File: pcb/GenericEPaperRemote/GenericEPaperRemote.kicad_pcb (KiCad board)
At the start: 2 copper layers, 190.5 x 61 mm, 113 parts, among them J1 Display, J2 speaker, J3 Prog, J4 JTAG, J5 Barrel_Jack, Q1 BC817, Q2 BC817, SW1 TactileSwitchSMD6x6, SW10 TactileSwitchSMD6x6, SW11 Rotary_Encoder_Switch, SW12 reset, SW13 bootloader, SW14 Conn_01x02_Male, SW2 TactileSwitchSMD6x6, SW3 TactileSwitchSMD6x6, SW4 TactileSwitchSMD6x6, SW5 TactileSwitchSMD6x6, SW6 TactileSwitchSMD6x6, SW7 TactileSwitchSMD6x6, SW8 TactileSwitchSMD6x6, SW9 TactileSwitchSMD6x6, U1 ESP32-WROVER-B_(16MB), U2 FT232RL, U3 NCP1117ST33T3G

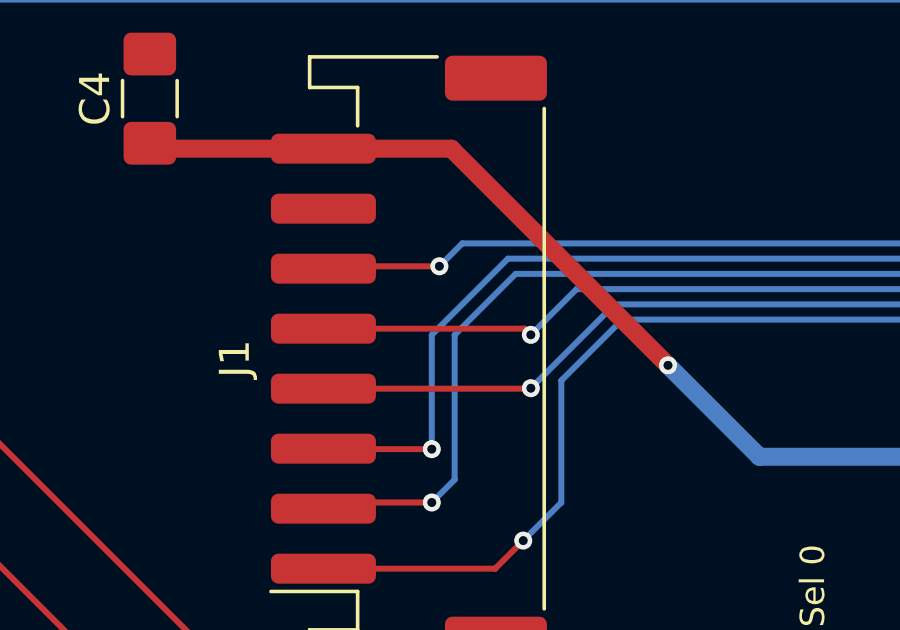
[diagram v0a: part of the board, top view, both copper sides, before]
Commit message: small changes
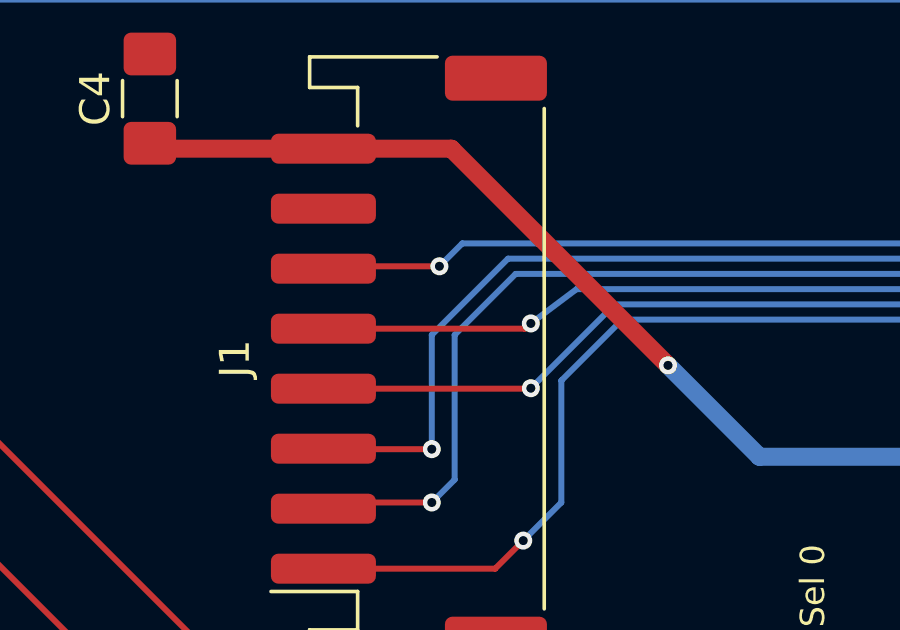
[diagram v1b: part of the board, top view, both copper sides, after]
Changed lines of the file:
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@@
     (38 B.Mask user)
     (39 F.Mask user)
-    (40 Dwgs.User user)
+    (40 Dwgs.User user hide)
     (41 Cmts.User user)
     (42 Eco1.User user)
@@
   (segment (start 135.66 101.6) (end 135.58 101.68) (width 0.2) (layer Front) (net 42))
   (segment (start 139.446 101.6) (end 135.66 101.6) (width 0.2) (layer Front) (net 42))
-  (via (at 142.494 103.886) (size 0.6) (drill 0.3) (layers Front Back) (net 43))
-  (segment (start 142.288 103.68) (end 142.494 103.886) (width 0.2) (layer Front) (net 43))
-  (segment (start 135.58 103.68) (end 142.288 103.68) (width 0.2) (layer Front) (net 43))
-  (segment (start 142.494 103.886) (end 144.018 102.362) (width 0.2) (layer Back) (net 43))
-  (segment (start 144.018 102.362) (end 197.72938 102.362) (width 0.2) (layer Back) (net 43))
   (segment (start 201.67138 98.42) (end 213.75 98.42) (width 0.2) (layer Back) (net 43))
   (segment (start 197.72938 102.362) (end 201.67138 98.42) (width 0.2) (layer Back) (net 43))
+  (segment (start 144.018 102.362) (end 197.72938 102.362) (width 0.2) (layer Back) (net 43))
+  (segment (start 142.494 103.505) (end 144.018 102.362) (width 0.2) (layer Back) (net 43))
+  (segment (start 142.288 103.68) (end 135.58 103.68) (width 0.2) (layer Front) (net 43))
+  (segment (start 142.494 103.505) (end 142.288 103.68) (width 0.2) (layer Front) (net 43))
+  (via (at 142.494 103.505) (size 0.6) (drill 0.3) (layers Front Back) (net 43))
   (via (at 142.494 105.664) (size 0.6) (drill 0.3) (layers Front Back) (net 44))
   (segment (start 142.478 105.68) (end 142.494 105.664) (width 0.2) (layer Front) (net 44))
@@
     (connect_pads (clearance 0.508))
     (min_thickness 0.254)
-    (fill (arc_segments 32) (thermal_gap 0.508) (thermal_bridge_width 0.508))
+    (fill yes (arc_segments 32) (thermal_gap 0.508) (thermal_bridge_width 0.508))
     (polygon
       (pts
@@
     (connect_pads (clearance 0.508))
     (min_thickness 0.254)
-    (fill (arc_segments 32) (thermal_gap 0.508) (thermal_bridge_width 0.508))
+    (fill yes (arc_segments 32) (thermal_gap 0.508) (thermal_bridge_width 0.508))
     (polygon
       (pts
